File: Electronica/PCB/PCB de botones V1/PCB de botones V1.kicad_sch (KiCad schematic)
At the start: 14 parts, among them J2 Conn_02x05_Counter_Clockwise, SW2 SW_Push, SW4 SW_Push, SW9 SW_SPST

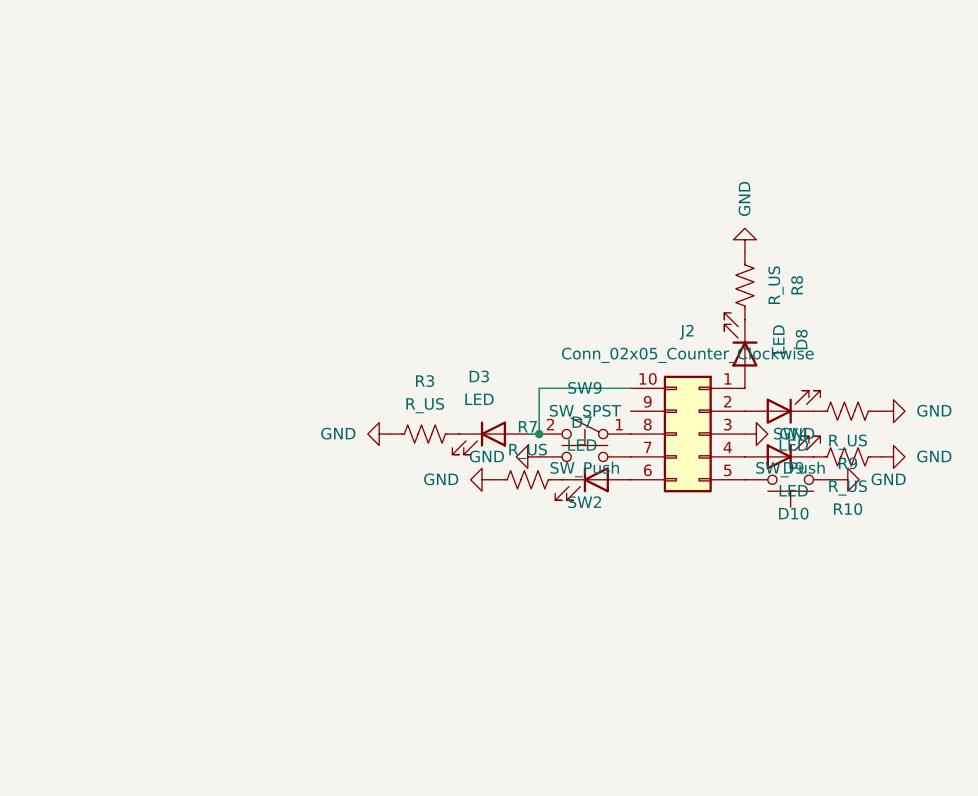
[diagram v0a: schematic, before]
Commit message: .
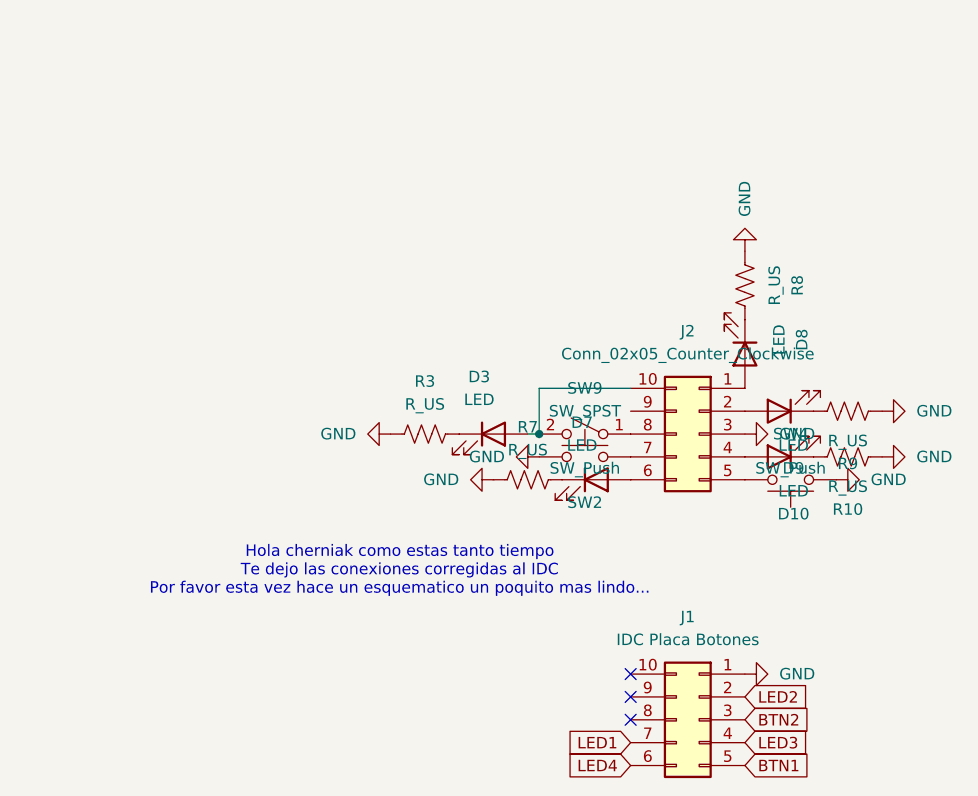
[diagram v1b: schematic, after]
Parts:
- added J1: IDC Placa Botones, Connector_IDC:IDC-Header_2x05_P2.54mm_Horizontal, symbol Connector_Generic:Conn_02x05_Counter_Clockwise
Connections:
- net GND: now also J1.1 (Pin_1)
- new net BTN1: J1.5 (Pin_5)
- new net BTN2: J1.3 (Pin_3)
- new net LED1: J1.7 (Pin_7)
- new net LED2: J1.2 (Pin_2)
- new net LED3: J1.4 (Pin_4)
- new net LED4: J1.6 (Pin_6)
- no-connect marks 0 -> 3
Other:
- note added: "Hola cherniak como estas tanto tiempo Te dejo las conexiones corregidas al IDC Por favor esta vez hace un esquematico un poquito mas lindo..."

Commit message: pcb de leds
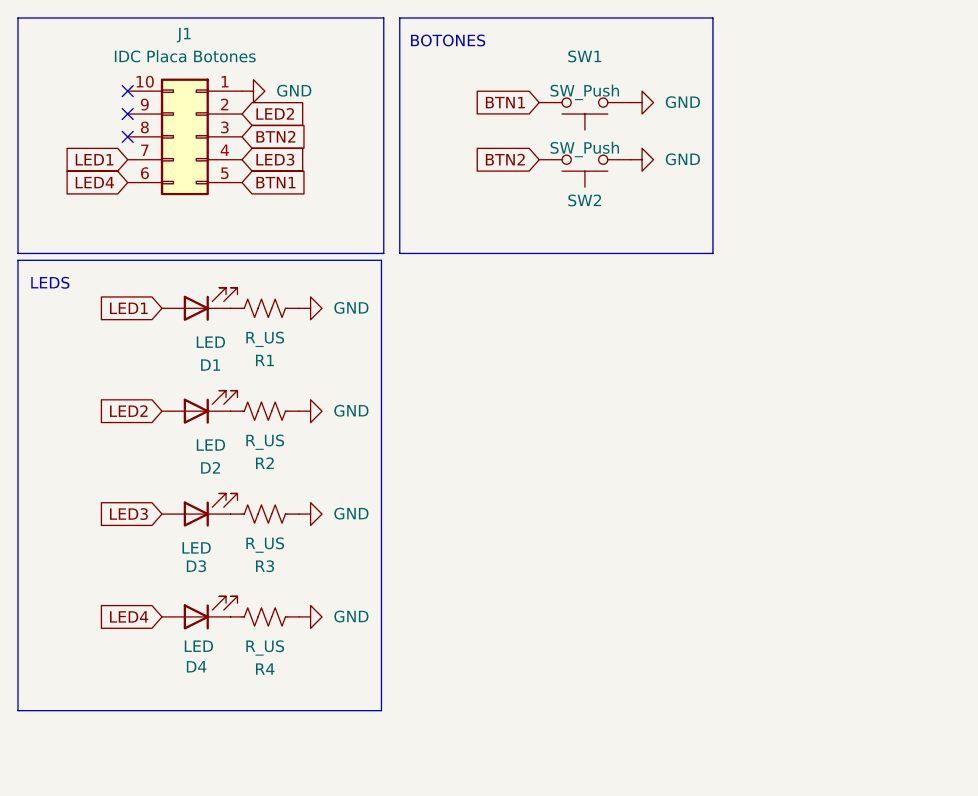
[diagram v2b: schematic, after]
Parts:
- removed D10, D7, D8, D9: LED, LED_THT:LED_D5.0mm, symbol Device:LED
- removed J2: Conn_02x05_Counter_Clockwise, Connector_IDC:IDC-Header_2x05_P2.54mm_Vertical, symbol Connector_Generic:Conn_02x05_Counter_Clockwise
- removed R10, R7, R8, R9: R_US, Resistor_THT:R_Axial_DIN0207_L6.3mm_D2.5mm_P10.16mm_Horizontal, symbol Device:R_US
- removed SW4: SW_Push, Button_Switch_THT:SW_PUSH_6mm, symbol Switch:SW_Push
- removed SW9: SW_SPST, Button_Switch_THT:SW_Slide_SPDT_Straight_CK_OS102011MS2Q, symbol Switch:SW_SPST
- added D1, D2, D4: LED, LED_THT:LED_D5.0mm, symbol Device:LED
- added R1, R2, R4: R_US, Resistor_THT:R_Axial_DIN0207_L6.3mm_D2.5mm_P10.16mm_Horizontal, symbol Device:R_US
- added SW1: SW_Push, Button_Switch_THT:SW_PUSH_6mm, symbol Switch:SW_Push
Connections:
- net BTN1: now also SW1.1
- net BTN2: now also SW2.1
- net GND: now also R1.1, R2.1, R4.1, SW1.2
- net LED1: now also D1.2 (A)
- net LED2: now also D2.2 (A)
- net LED3: now also D3.2 (A)
- net LED4: now also D4.2 (A)
- new net: D2.1 (K), R2.2
- new net: D4.1 (K), R4.2
- new net: D1.1 (K), R1.2
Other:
- note added: "BOTONES"
- note added: "LEDS"
- note removed: "Hola cherniak como estas tanto tiempo Te dejo las conexiones corregidas al IDC Por favor esta vez hace un esquematico un poquito mas lindo..."
- moved on the sheet: J1
